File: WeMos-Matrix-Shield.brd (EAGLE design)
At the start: 45.1 x 48.9 mm, 18 parts, among them CN1 1X4-BIG, J2 POWER_JACKPTH, U1 LDR, U2 DS18B20, X1 SPTAF_25.0MM

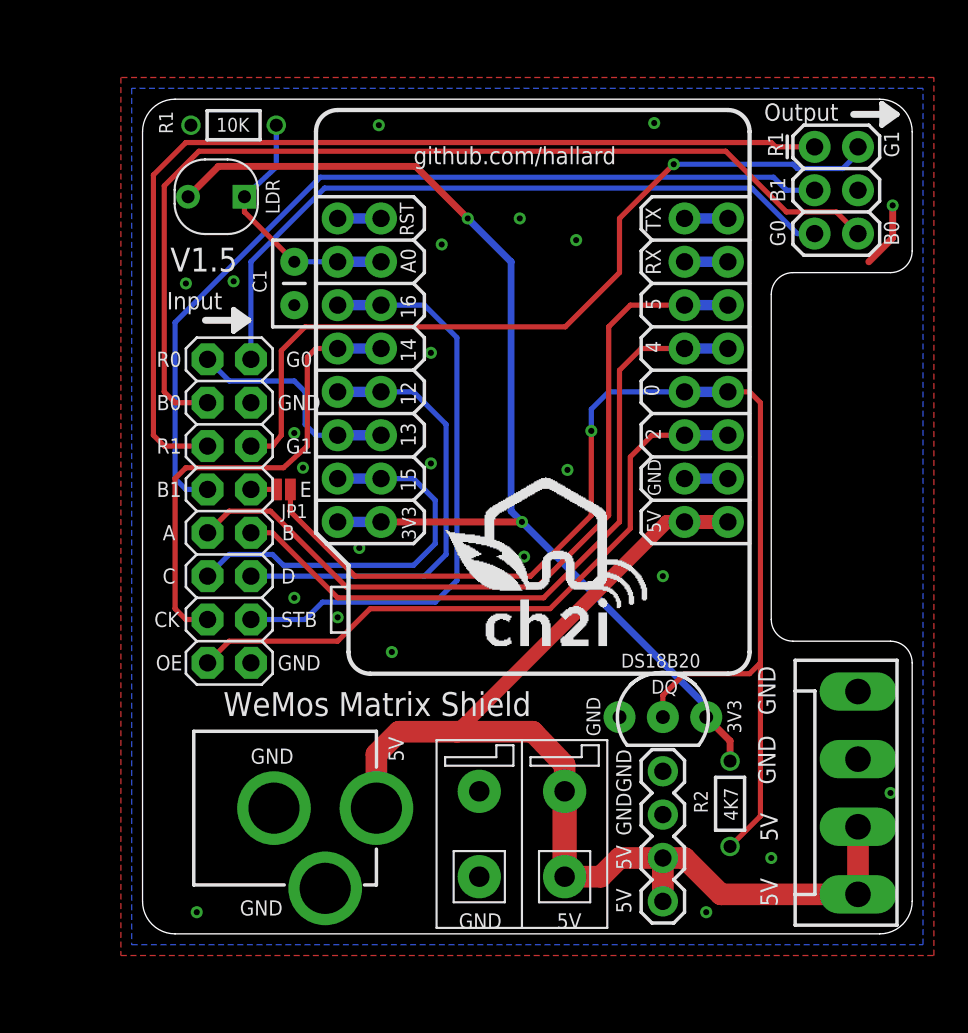
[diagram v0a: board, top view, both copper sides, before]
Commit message: Updated to V1.6
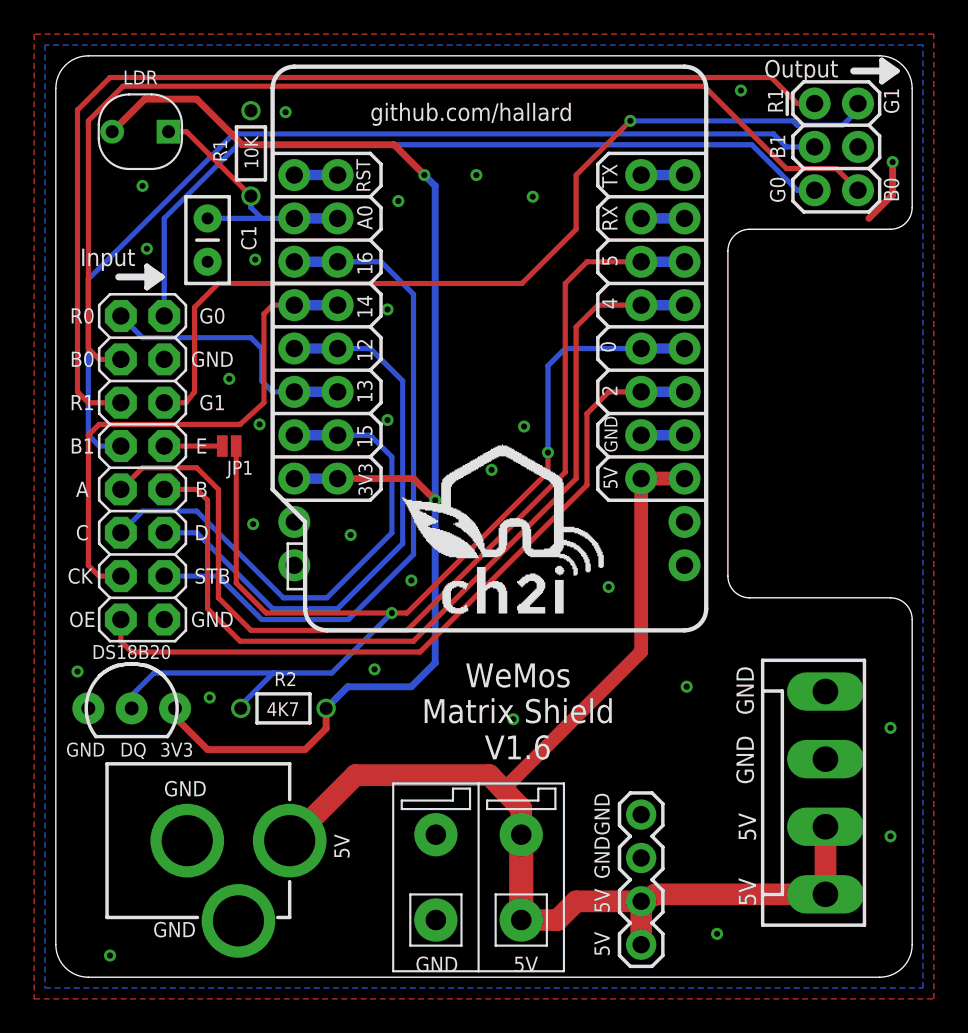
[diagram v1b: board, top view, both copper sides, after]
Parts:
- added VIN1, VIN2, VIN3, VIN4: PADNORMAL, _c2h:PAD
- moved U2 31.1 mm to (9.53, 15.7)
- moved R2 26.8 mm to (18.4, 15.7), turned to 0 degrees
- moved U1 5.85 mm to (10.0, 49.5)
- moved C1 5.68 mm to (14.0, 44.5)
- moved JP2 5.68 mm to (8.89, 38.7)
- moved J2 5.43 mm to (5.08, 8.00)
- moved JP1 4.07 mm to (15.2, 31.1)
- moved JP4 3.59 mm to (41.9, 47.0)
- moved X1 3.59 mm to (29.8, 6.35)
- moved JP3 3.59 mm to (19.1, 47.0)
- moved JP7 3.59 mm to (21.6, 47.0)
- moved JP8 3.59 mm to (39.4, 47.0)
- moved U$3 3.18 mm to (31.9, 24.3)
- moved CN1 2.84 mm to (39.4, 1.91)
- moved J1 2.54 mm to (49.5, 51.2)
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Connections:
- new net SD3: VIN4.1
- new net SDO: VIN2.1
- new net TCK: VIN3.1
- new net TDO: VIN1.1
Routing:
- net 3V3: track 67.3 -> 77.9 mm
- net B: track 40.8 -> 51.2 mm
- net A: track 46.2 -> 56.6 mm
- net DQ: track 73.3 -> 65.9 mm, vias 1 -> 2
- net D: track 29.3 -> 36.6 mm
- net C: track 26.0 -> 33.3 mm
- net B0: track 58.3 -> 64.0 mm
- net R1: track 58.3 -> 63.9 mm
- net STB: track 37.5 -> 42.8 mm
- net G0: track 41.6 -> 46.7 mm
- net B1: track 52.6 -> 57.7 mm
- net G1: track 48.1 -> 53.1 mm
- net OE: track 38.5 -> 43.3 mm
- net R0: track 13.1 -> 15.7 mm
- net CLK: track 28.0 -> 30.6 mm
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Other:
- board size 45.1 x 48.9 mm -> 50.2 x 54 mm
- board text added: "V1.6"
- board text added: "WeMos Matrix Shield V1.6"
- board text removed: "V1.5"
- board text removed: "WeMos Matrix Shield V1.5"
